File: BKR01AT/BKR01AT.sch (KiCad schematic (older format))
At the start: 46 parts

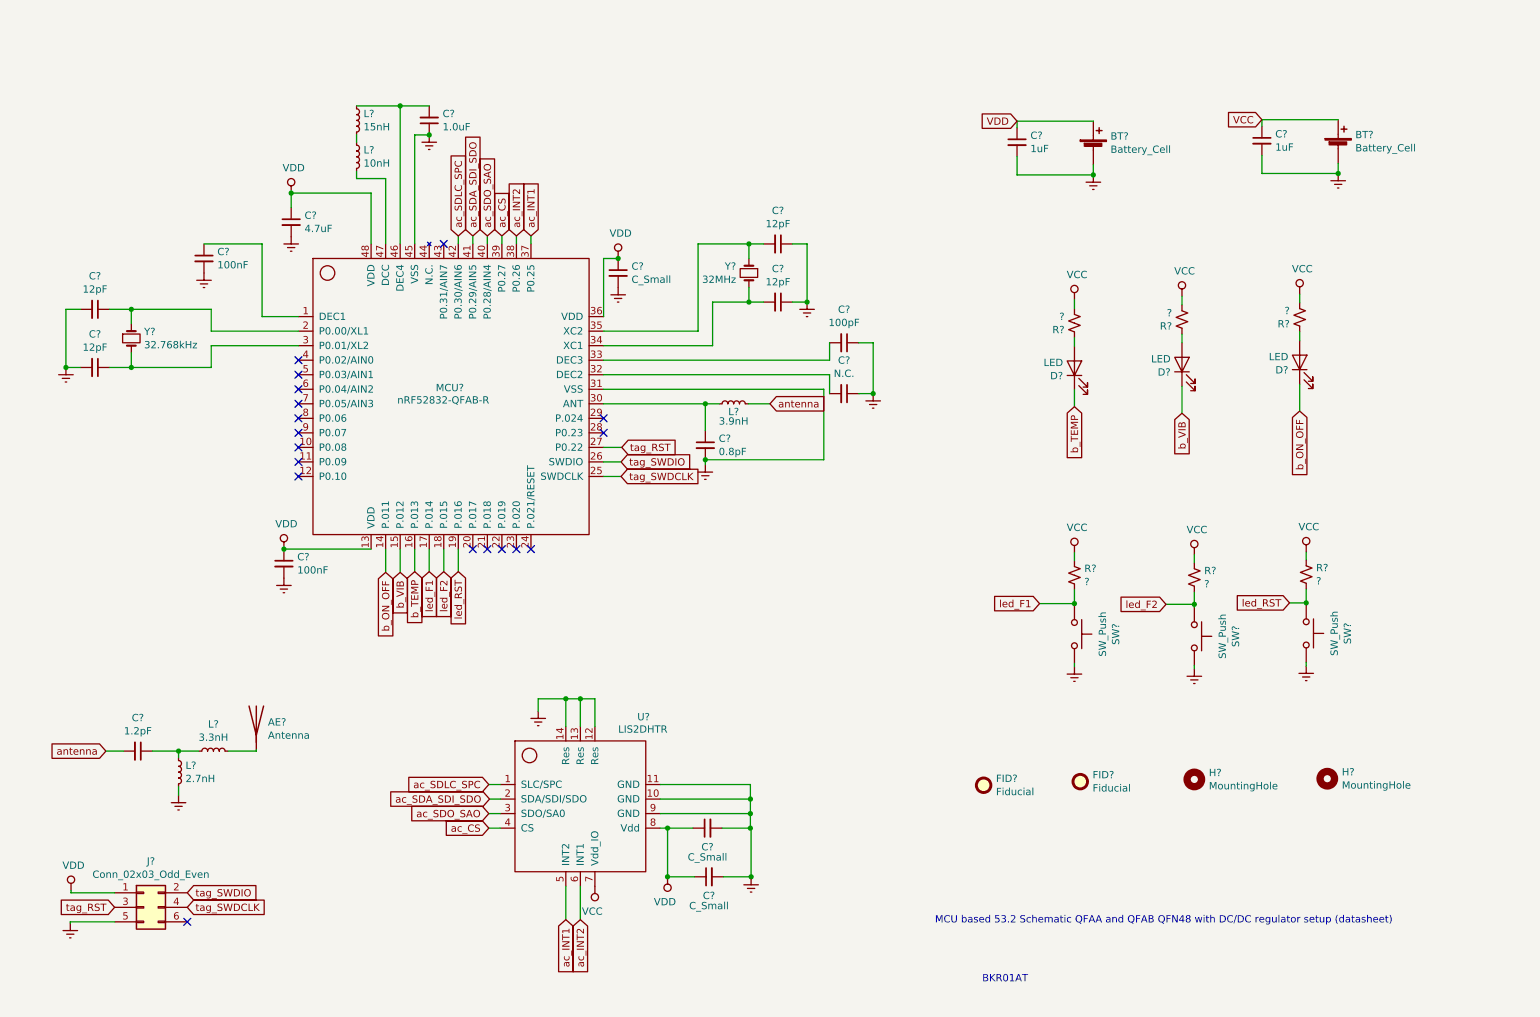
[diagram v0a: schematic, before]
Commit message: organizando o esquemático
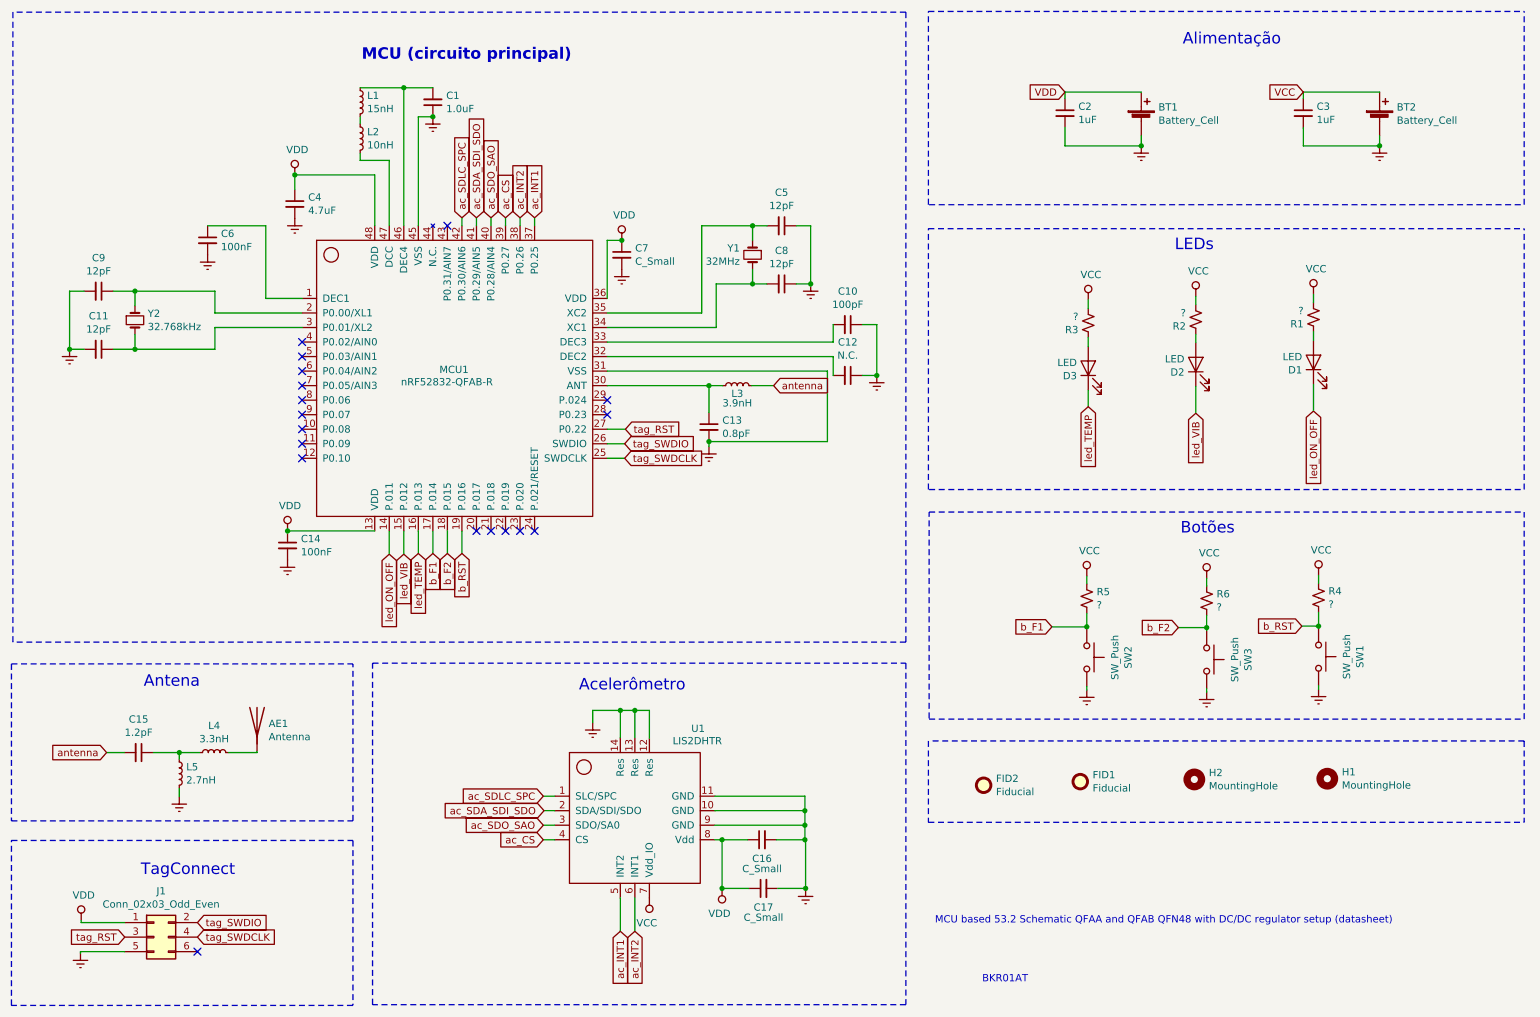
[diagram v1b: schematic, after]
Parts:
- gave numbers to parts that had none: 46
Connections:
- net b_ON_OFF renamed led_ON_OFF
- net b_TEMP renamed led_TEMP
- net b_VIB renamed led_VIB
- net led_F1 renamed b_F1
- net led_F2 renamed b_F2
- net led_RST renamed b_RST
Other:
- note added: "Acelerômetro"
- note added: "Alimentação"
- note added: "Antena"
- note added: "Botões"
- note added: "LEDs"
- note added: "MCU (circuito principal)"
- note added: "TagConnect"
- moved on the sheet: BT1, BT2, C1, C10, C11, C12, C13, C14, C16, C17, C2, C3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
